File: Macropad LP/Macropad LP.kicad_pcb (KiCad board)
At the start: 2 copper layers, 54 x 85.6 mm, 11 parts, among them J1 switch 1, J2 switch 2, J3 switch 3, J4 switch 4, J5 switch 5, J6 switch 6, J7 switch 7, J8 switch 8, U1 Pico

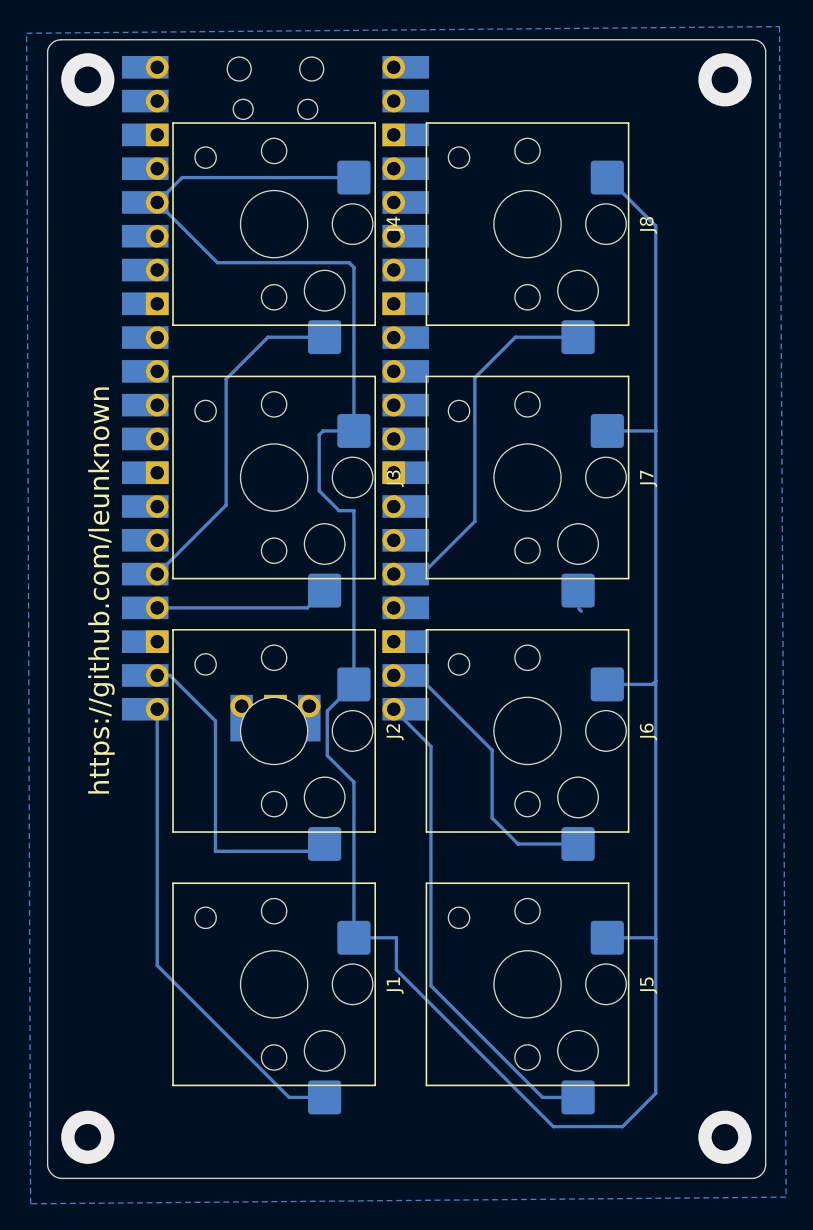
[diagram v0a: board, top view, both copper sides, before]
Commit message: Add files via upload
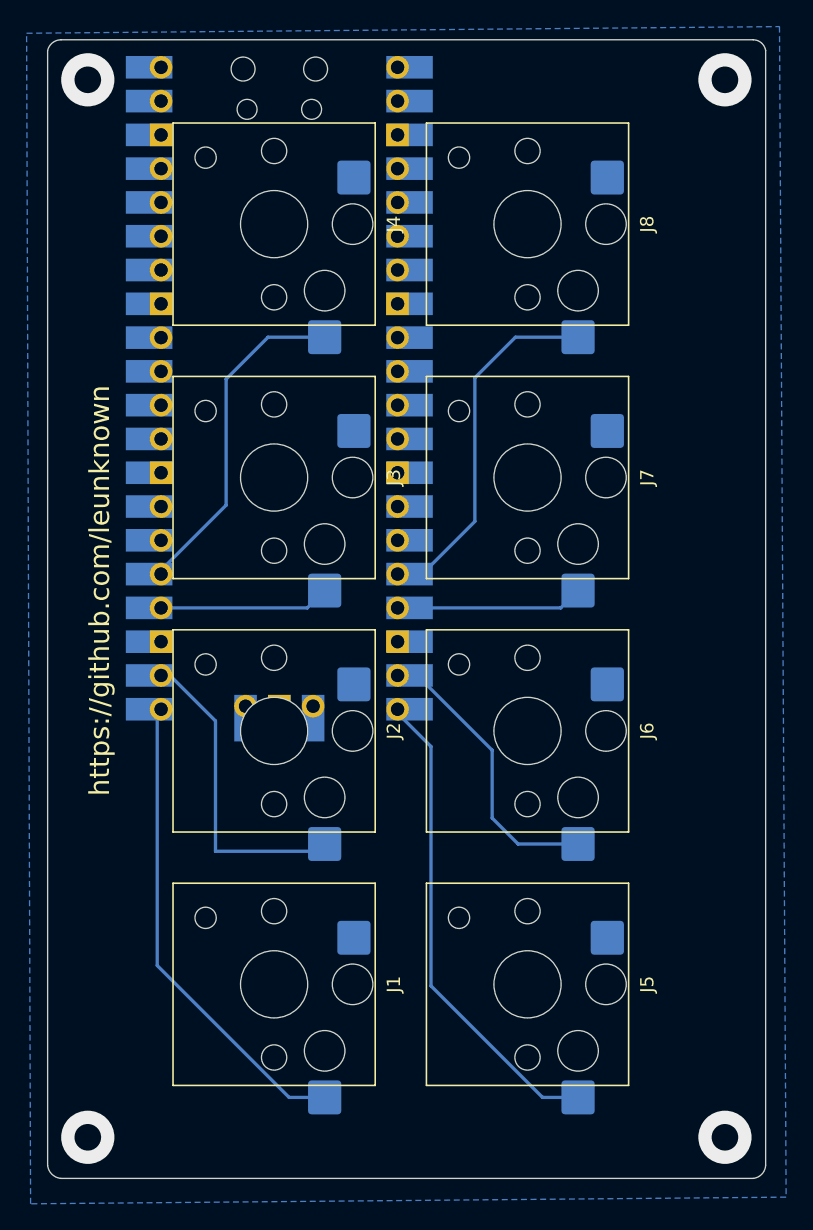
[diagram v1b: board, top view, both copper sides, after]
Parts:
- moved U1 0.29 mm to (86.0, 46.4)
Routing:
- net Out: track 201.0 -> 0.00 mm
- net Net-(J7-Pad2): track 0.27 -> 14.4 mm
- added copper zone on B.Cu, net Out
- removed copper zone on B.Cu, net (none)
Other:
- board text added: "Macrocard-LP v1.2 Theo Tang ©2022"
- board text removed: "Theo Tang ©2022"
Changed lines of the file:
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@@
   )
   (footprint "MCU_RaspberryPi_and_Boards:RPi_Pico_SMD_TH" (layer "B.Cu")
-    (at 85.71 46.39 180)
+    (at 86 46.39 180)
     (descr "Through hole straight pin header, 2x20, 2.54mm pitch, double rows")
     (tags "Through hole pin header THT 2x20 2.54mm double row")
@@
   (gr_line (start 121.62 20.19) (end 69.58 20.19) (layer "Edge.Cuts") (width 0.1))
   (gr_arc (start 122.56 104.79) (mid 122.276942 105.465726) (end 121.62 105.79) (layer "Edge.Cuts") (width 0.1))
-  (gr_text "Theo Tang\n©2022" (at 71.4 99.2 90) (layer "B.SilkS")
-    (effects (font (size 1 1) (thickness 0.15)) (justify right mirror))
+  (gr_text "Macrocard-LP v1.2\nTheo Tang\n©2022" (at 73 97.4 90) (layer "B.SilkS")
+    (effects (font (size 1.5 1.5) (thickness 0.3)) (justify right mirror))
   )
   (gr_text "https://github.com/leunknown" (at 72.5 61.6 90) (layer "F.SilkS")
     (effects (font (size 1.5 1.5) (thickness 0.3)))
   )
+  (dimension (type aligned) (layer "Dwgs.User")
+    (pts (xy 69.58 20.19) (xy 69.58 105.79))
+    (height 2.38)
+    (gr_text "85.6000 mm" (at 66.05 62.99 90) (layer "Dwgs.User")
+      (effects (font (size 1 1) (thickness 0.15)))
+    )
+    (format (units 3) (units_format 1) (precision 4))
+    (style (thickness 0.15) (arrow_length 1.27) (text_position_mode 0) (extension_height 0.58642) (extension_offset 0.5) keep_text_aligned)
+  )
+  (dimension (type aligned) (layer "Dwgs.User")
+    (pts (xy 68.58 104.819419) (xy 122.56 104.79))
+    (height 3.809803)
+    (gr_text "53.9800 mm" (at 95.571449 107.464512 0.03122502917) (layer "Dwgs.User")
+      (effects (font (size 1 1) (thickness 0.15)))
+    )
+    (format (units 3) (units_format 1) (precision 4))
+    (style (thickness 0.15) (arrow_length 1.27) (text_position_mode 0) (extension_height 0.58642) (extension_offset 0.5) keep_text_aligned)
+  )
   (via (at 71.6 23.2) (size 4) (drill 2) (layers "F.Cu" "B.Cu") (free) (net 0))
   (via (at 71.6 102.7) (size 4) (drill 2) (layers "F.Cu" "B.Cu") (free) (net 0))
   (via (at 119.5 102.7) (size 4) (drill 2) (layers "F.Cu" "B.Cu") (free) (net 0))
   (via (at 119.5 23.2) (size 4) (drill 2) (layers "F.Cu" "B.Cu") (free) (net 0))
-  (segment (start 91.6075 68.65) (end 91.6075 55.5925) (width 0.25) (layer "B.Cu") (net 16))
-  (segment (start 89.3 49.6) (end 91.6075 49.6) (width 0.25) (layer "B.Cu") (net 16))
-  (segment (start 91.6075 87.7) (end 91.6075 76.0075) (width 0.25) (layer "B.Cu") (net 16))
-  (segment (start 106.6 101.9) (end 111.8 101.9) (width 0.25) (layer "B.Cu") (net 16))
-  (segment (start 91.6075 49.6) (end 91.6075 37.3075) (width 0.25) (layer "B.Cu") (net 16))
-  (segment (start 114.3 99.4) (end 114.3 87.8) (width 0.25) (layer "B.Cu") (net 16))
-  (segment (start 78.69 30.55) (end 91.6075 30.55) (width 0.25) (layer "B.Cu") (net 16))
-  (segment (start 94.8 87.7) (end 94.8 90.1) (width 0.25) (layer "B.Cu") (net 16))
-  (segment (start 91.249521 36.949521) (end 81.349521 36.949521) (width 0.25) (layer "B.Cu") (net 16))
-  (segment (start 91.6075 76.0075) (end 89.607979 74.007979) (width 0.25) (layer "B.Cu") (net 16))
-  (segment (start 89 49.9) (end 89.3 49.6) (width 0.25) (layer "B.Cu") (net 16))
-  (segment (start 89.607979 70.649521) (end 91.6075 68.65) (width 0.25) (layer "B.Cu") (net 16))
-  (segment (start 91.6075 37.3075) (end 91.249521 36.949521) (width 0.25) (layer "B.Cu") (net 16))
-  (segment (start 114.3 34.1925) (end 110.6575 30.55) (width 0.25) (layer "B.Cu") (net 16))
-  (segment (start 94.8 90.1) (end 106.6 101.9) (width 0.25) (layer "B.Cu") (net 16))
-  (segment (start 114.3 49.6) (end 114.3 34.1925) (width 0.25) (layer "B.Cu") (net 16))
-  (segment (start 114.3 68.4) (end 114.3 49.6) (width 0.25) (layer "B.Cu") (net 16))
-  (segment (start 110.6575 68.65) (end 114.05 68.65) (width 0.25) (layer "B.Cu") (net 16))
-  (segment (start 90.4925 55.5925) (end 89 54.1) (width 0.25) (layer "B.Cu") (net 16))
-  (segment (start 114.05 68.65) (end 114.3 68.4) (width 0.25) (layer "B.Cu") (net 16))
-  (segment (start 89 54.1) (end 89 49.9) (width 0.25) (layer "B.Cu") (net 16))
-  (segment (start 114.3 87.8) (end 114.3 68.4) (width 0.25) (layer "B.Cu") (net 16))
-  (segment (start 89.607979 74.007979) (end 89.607979 70.649521) (width 0.25) (layer "B.Cu") (net 16))
-  (segment (start 76.82 32.42) (end 78.69 30.55) (width 0.25) (layer "B.Cu") (net 16))
-  (segment (start 111.8 101.9) (end 114.3 99.4) (width 0.25) (layer "B.Cu") (net 16))
-  (segment (start 91.6075 87.7) (end 94.8 87.7) (width 0.25) (layer "B.Cu") (net 16))
-  (segment (start 110.6575 49.6) (end 114.3 49.6) (width 0.25) (layer "B.Cu") (net 16))
-  (segment (start 91.6075 55.5925) (end 90.4925 55.5925) (width 0.25) (layer "B.Cu") (net 16))
-  (segment (start 81.349521 36.949521) (end 76.82 32.42) (width 0.25) (layer "B.Cu") (net 16))
-  (segment (start 114.2 87.7) (end 114.3 87.8) (width 0.25) (layer "B.Cu") (net 16))
-  (segment (start 110.6575 87.7) (end 114.2 87.7) (width 0.25) (layer "B.Cu") (net 16))
   (segment (start 86.734343 99.7) (end 89.4075 99.7) (width 0.25) (layer "B.Cu") (net 17))
   (segment (start 76.82 89.785657) (end 86.734343 99.7) (width 0.25) (layer "B.Cu") (net 17))
@@
   (segment (start 97.4 73.32) (end 97.4 91.315657) (width 0.25) (layer "B.Cu") (net 22))
   (segment (start 97.4 91.315657) (end 105.784343 99.7) (width 0.25) (layer "B.Cu") (net 22))
-  (segment (start 108.51 62.96) (end 108.7 63.15) (width 0.25) (layer "B.Cu") (net 24))
+  (segment (start 94.6 62.9) (end 107.1575 62.9) (width 0.25) (layer "B.Cu") (net 24))
+  (segment (start 107.1575 62.9) (end 108.4575 61.6) (width 0.25) (layer "B.Cu") (net 24))
   (segment (start 94.99 60.42) (end 96.599022 60.42) (width 0.25) (layer "B.Cu") (net 25))
   (segment (start 94.6 60.36) (end 96.74 60.36) (width 0.25) (layer "B.Cu") (net 25))
@@
   (segment (start 94.99 68.04) (end 96.599022 68.04) (width 0.25) (layer "B.Cu") (net 36))
   (segment (start 102 73.6) (end 102 78.7) (width 0.25) (layer "B.Cu") (net 36))
-  (zone (net 0) (net_name "") (layer "B.Cu") (hatch edge 0.508)
+  (zone (net 16) (net_name "Out") (layer "B.Cu") (hatch edge 0.508)
     (connect_pads (clearance 0.508))
     (min_thickness 0.254) (filled_areas_thickness no)
